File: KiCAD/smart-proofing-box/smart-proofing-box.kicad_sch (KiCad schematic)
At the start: 8 parts, among them J1 Screw_Terminal_01x02, J2 USB_C_Receptacle, SW1 SW_Push

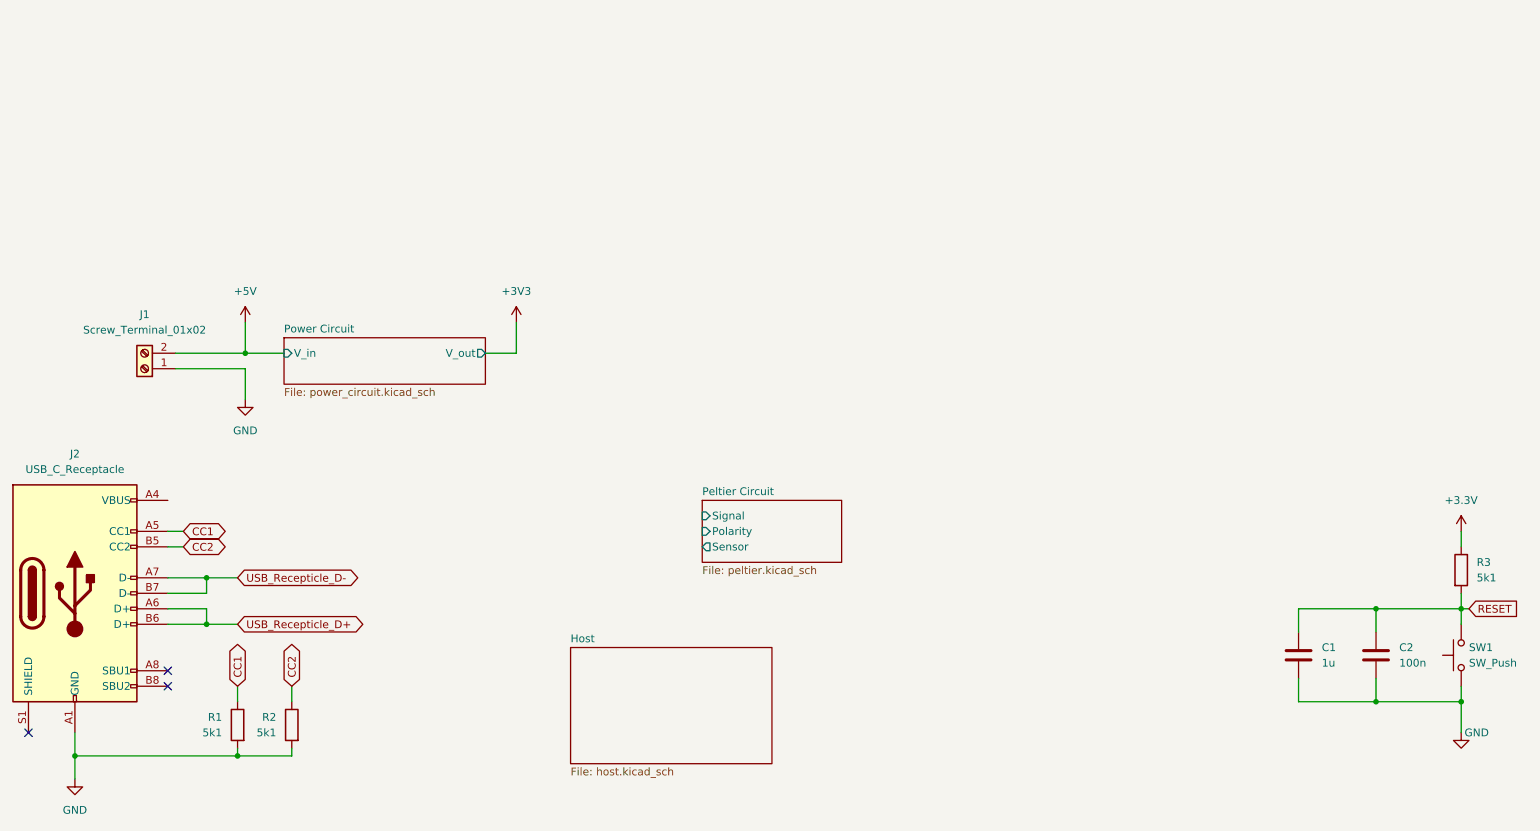
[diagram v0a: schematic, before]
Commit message: continued sketching rough design
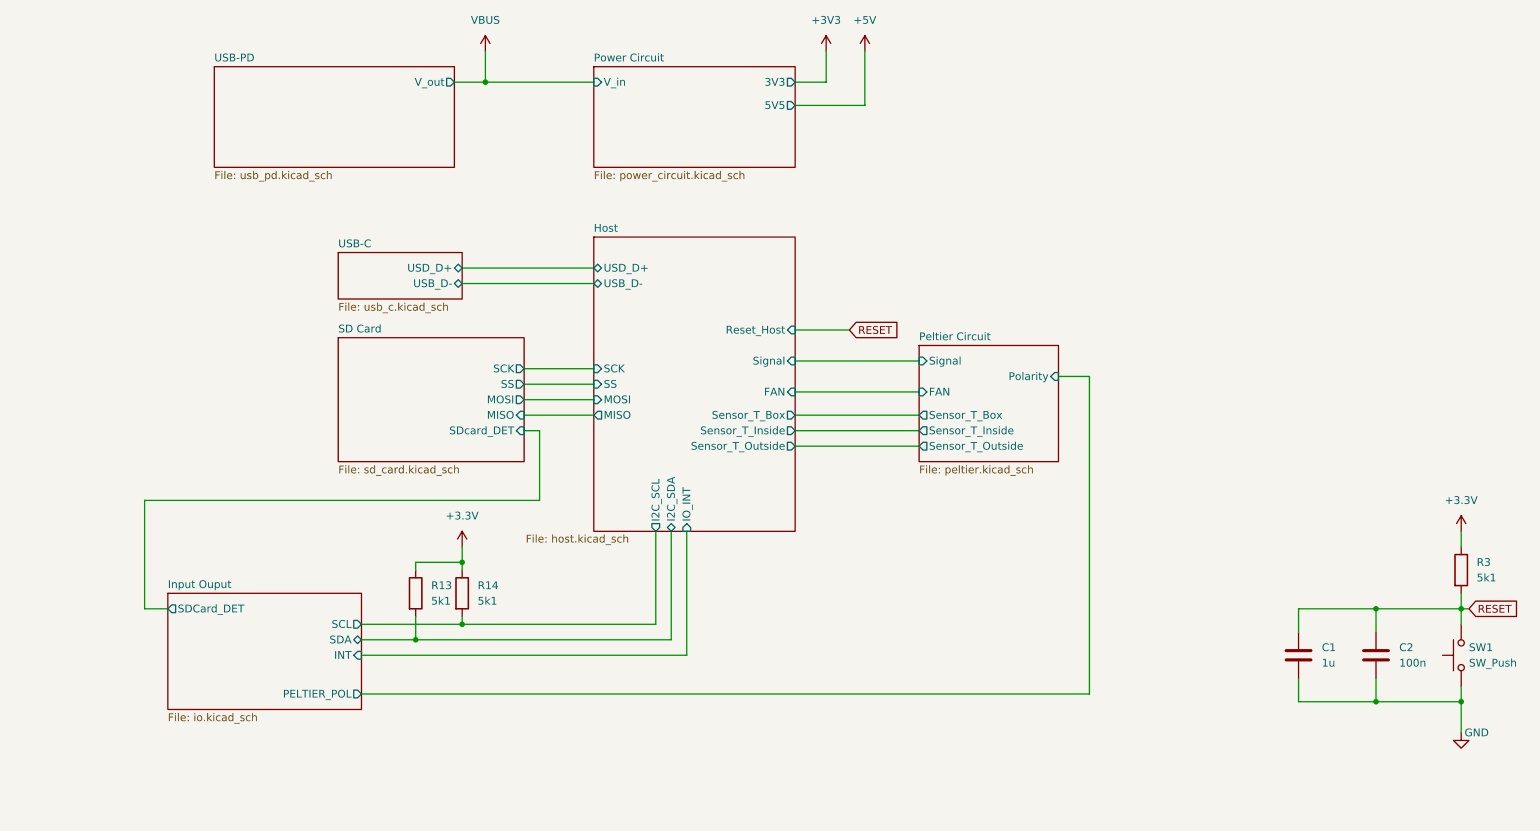
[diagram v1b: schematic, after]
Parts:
- removed J1: Screw_Terminal_01x02, symbol Connector:Screw_Terminal_01x02
- removed J2: USB_C_Receptacle, Prj_Connectors_USB:USB_C_Receptacle_SHOU_HAN_TYPE_C_16P_CB1.6_073, symbol Connector:USB_C_Receptacle_USB2.0
- removed R1, R2: 5k1, Resistor_SMD:R_0402_1005Metric_Pad0.72x0.64mm_HandSolder, symbol Device:R
- added R13, R14: 5k1, Resistor_SMD:R_0402_1005Metric_Pad0.72x0.64mm_HandSolder, symbol Device:R
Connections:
- net +3.3V: now also R13.1, R14.1
- new net Host/I2C_SCL: R14.2
- new net Host/I2C_SDA: R13.2
- no-connect marks 3 -> 0
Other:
- added sheet Input Ouput (io.kicad_sch)
- added sheet SD Card (sd_card.kicad_sch)
- added sheet USB-C (usb_c.kicad_sch)
- added sheet USB-PD (usb_pd.kicad_sch)
- sheet Host ports: added FAN, I2C_SCL, I2C_SDA, IO_INT, MISO, MOSI, Reset_Host, SCK, SS, Sensor_T_Box, Sensor_T_Inside, Sensor_T_Outside, Signal, USB_D-, USD_D+; removed none
- sheet Peltier Circuit ports: added FAN, Sensor_T_Box, Sensor_T_Inside, Sensor_T_Outside; removed Sensor
- sheet Power Circuit ports: added 3V3, 5V5; removed V_out
